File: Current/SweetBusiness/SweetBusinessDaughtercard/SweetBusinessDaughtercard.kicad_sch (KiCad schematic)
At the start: 8 parts, among them K10 Jump Out, K11 Jump Out, K12 Jump Out, K13 Jump Out, SW1 SW_SPDT, SW2 SW_SPDT, SW3 SW_SPDT, SW4 SW_SPDT

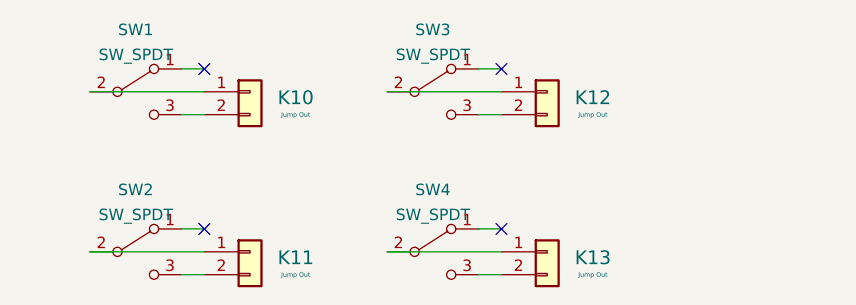
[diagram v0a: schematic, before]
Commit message: Nice changelog, idiot.
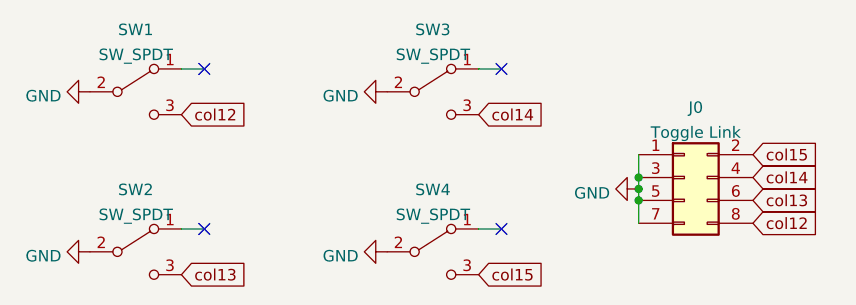
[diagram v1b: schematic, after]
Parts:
- removed K10, K11, K12, K13: Jump Out, Connector_PinSocket_2.54mm:PinSocket_1x02_P2.54mm_Vertical, symbol Connector_Generic:Conn_01x02
- added J0: Toggle Link, Connector_PinHeader_2.54mm:PinHeader_2x04_P2.54mm_Vertical, symbol Connector_Generic:Conn_02x04_Odd_Even
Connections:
- net GND: now reaches SW2.2 (B)
- net GND: now also SW1.2 (B), SW3.2 (B), SW4.2 (B), J0.1 (Pin_1), J0.3 (Pin_3), J0.5 (Pin_5), J0.7 (Pin_7)
- net col13: now reaches SW2.3 (C)
- net col13: now also J0.6 (Pin_6)
- net col14: now reaches SW3.3 (C)
- net col14: now also J0.4 (Pin_4)
- net col12: now reaches SW1.3 (C)
- net col12: now also J0.8 (Pin_8)
- net col15: now reaches SW4.3 (C)
- net col15: now also J0.2 (Pin_2)
